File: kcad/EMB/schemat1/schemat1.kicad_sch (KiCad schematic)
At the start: 4 parts, among them IC1 ESP32-C6-WROOM-1-N8, U1 ER_OLEDM0.91_1x-I2C

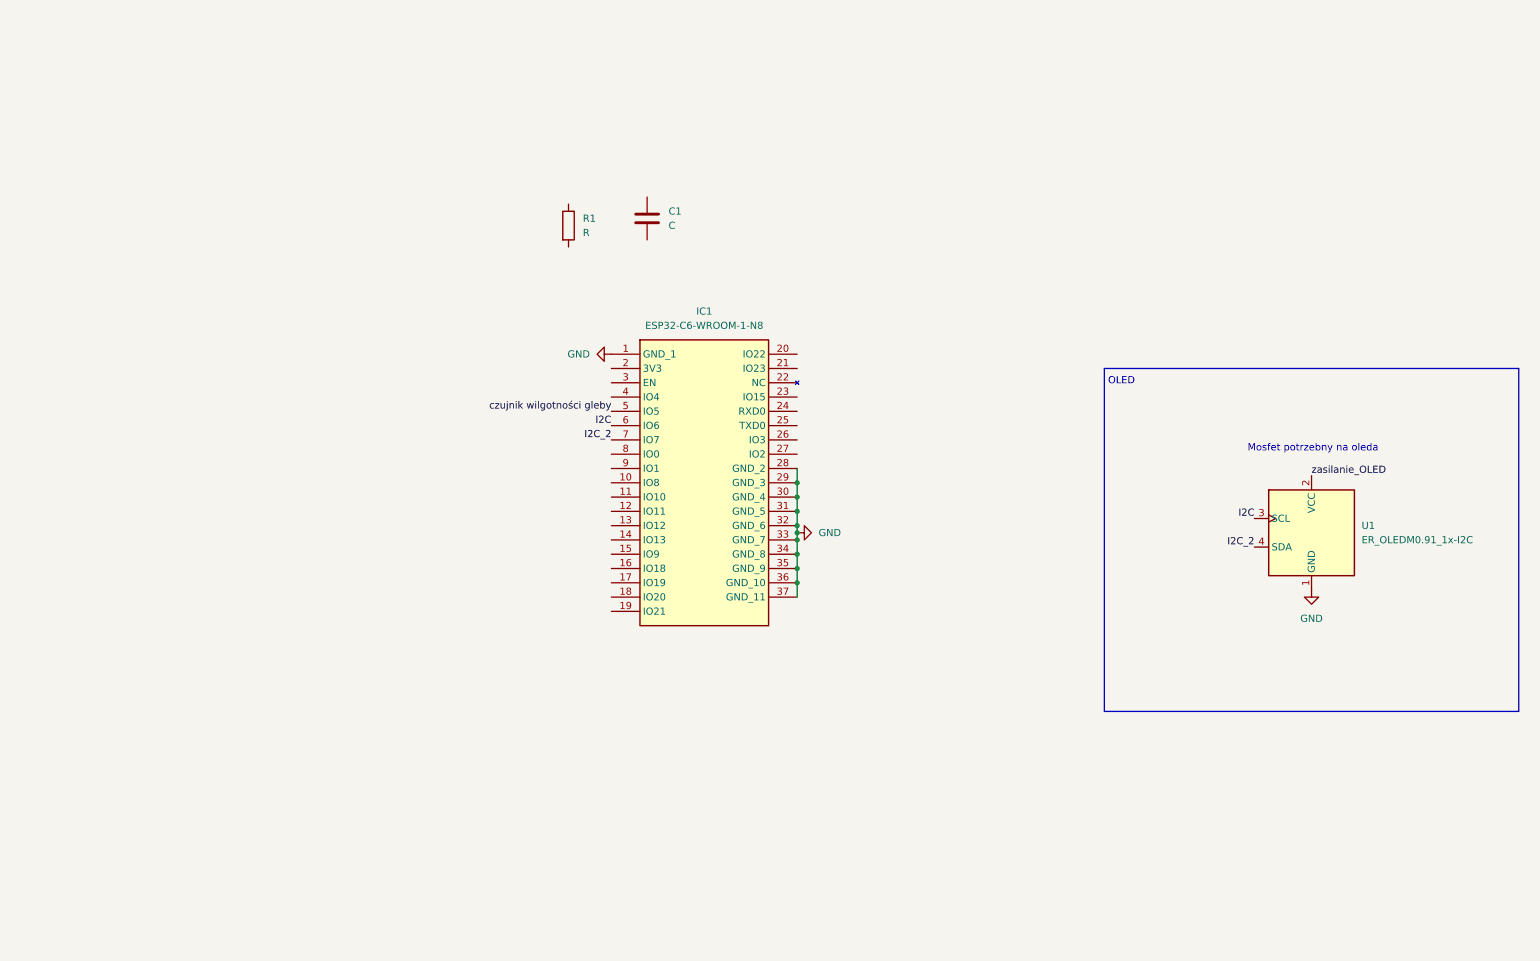
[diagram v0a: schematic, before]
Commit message: edit
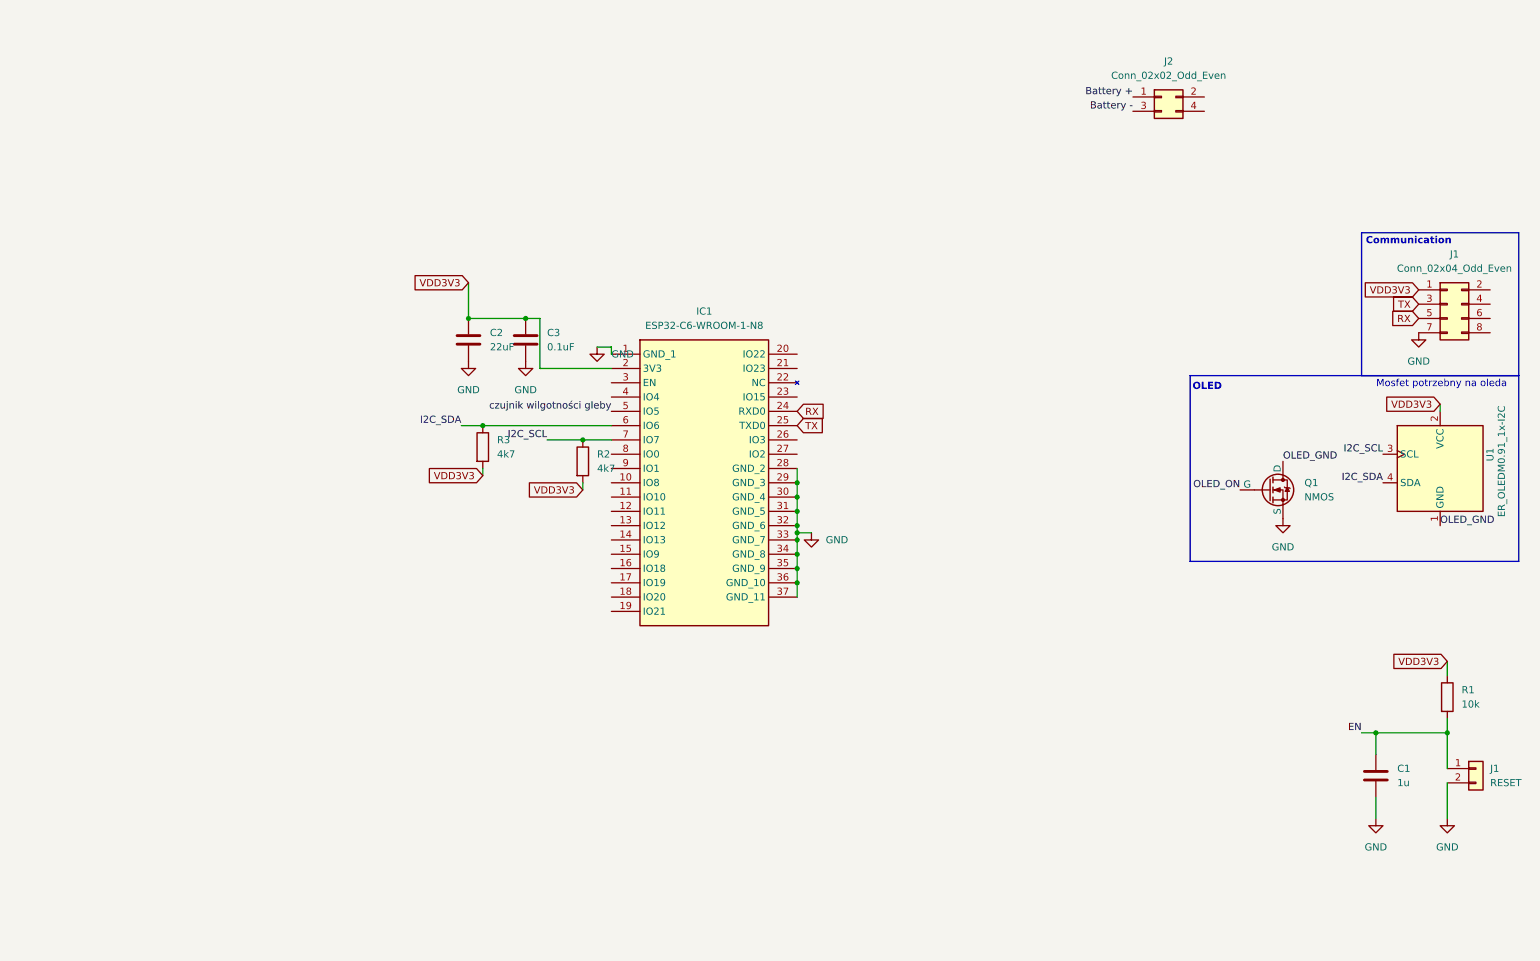
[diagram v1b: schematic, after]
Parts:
- added C2: 22uF, symbol Device:C
- added C3: 0.1uF, symbol Device:C
- added J1: RESET, symbol Connector_Generic:Conn_01x02
- added J1: Conn_02x04_Odd_Even, symbol Connector_Generic:Conn_02x04_Odd_Even
- added J2: Conn_02x02_Odd_Even, symbol Connector_Generic:Conn_02x02_Odd_Even
- added Q1: NMOS, symbol Simulation_SPICE:NMOS
- added R2, R3: 4k7, symbol Device:R
- C1: value C -> 1u
- R1: value R -> 10k
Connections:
- net zasilanie_OLED is gone; now on net VDD3V3: U1.2 (VCC)
- net GND: now also C1.2, C2.2, C3.2, J1.2 (Pin_2), J1.7 (Pin_7), Q1.3 (S); no longer U1.1 (GND)
- net VDD3V3: now reaches R1.1
- net VDD3V3: now also IC1.2 (3V3), C2.1, C3.1, J1.1 (Pin_1), R2.2, R3.2
- net EN: now reaches R1.2
- net EN: now also C1.1, J1.1 (Pin_1)
- net RX: now reaches IC1.24 (RXD0)
- net RX: now also J1.5 (Pin_5)
- net TX: now reaches IC1.25 (TXD0)
- net TX: now also J1.3 (Pin_3)
- net I2C renamed I2C_SCL
- net I2C_SCL: now also IC1.7 (IO7), R2.1; no longer IC1.6 (IO6)
- net I2C_2 renamed I2C_SDA
- net I2C_SDA: now also IC1.6 (IO6), R3.1; no longer IC1.7 (IO7)
- new net Battery +: J2.1 (Pin_1)
- new net Battery -: J2.3 (Pin_3)
- new net OLED_GND: Q1.1 (D), U1.1 (GND)
- new net OLED_ON: Q1.2 (G)
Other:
- note added: "Communication"
- moved on the sheet: U1

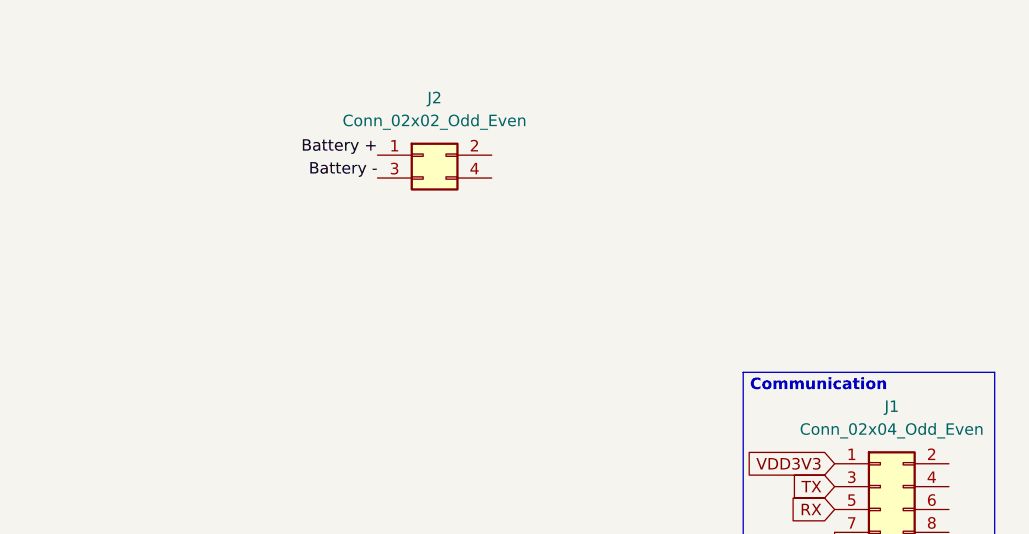
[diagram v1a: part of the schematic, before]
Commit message: update
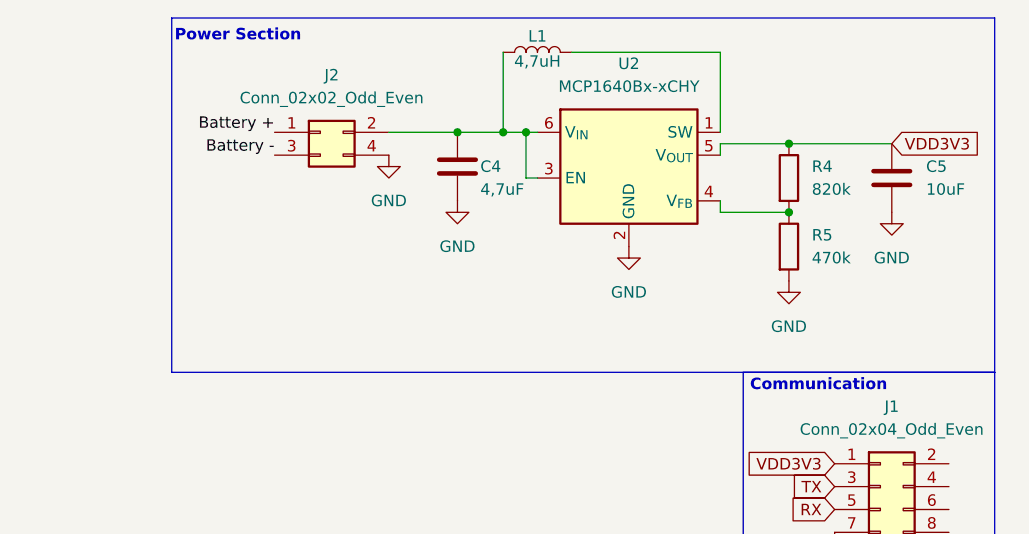
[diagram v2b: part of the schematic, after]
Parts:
- added C4: 4,7uF, symbol Device:C
- added C5: 10uF, symbol Device:C
- added L1: 4,7uH, symbol Device:L
- added R4: 820k, symbol Device:R
- added R5: 470k, symbol Device:R
- added U2: MCP1640Bx-xCHY, Package_TO_SOT_SMD:SOT-23-6, symbol Regulator_Switching:MCP1640Bx-xCHY
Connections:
- net GND: now also J2.4 (Pin_4), C4.2, C5.2, R5.2, U2.2 (GND)
- net VDD3V3: now also C5.1, R4.1, U2.5 (V_{OUT})
- net at J2.2 (Pin_2): now also C4.1, L1.1, U2.3 (EN), U2.6 (V_{IN})
- new net: R4.2, R5.1, U2.4 (V_{FB})
- new net: L1.2, U2.1 (SW)
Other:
- note added: "Power Section"
- moved on the sheet: J2

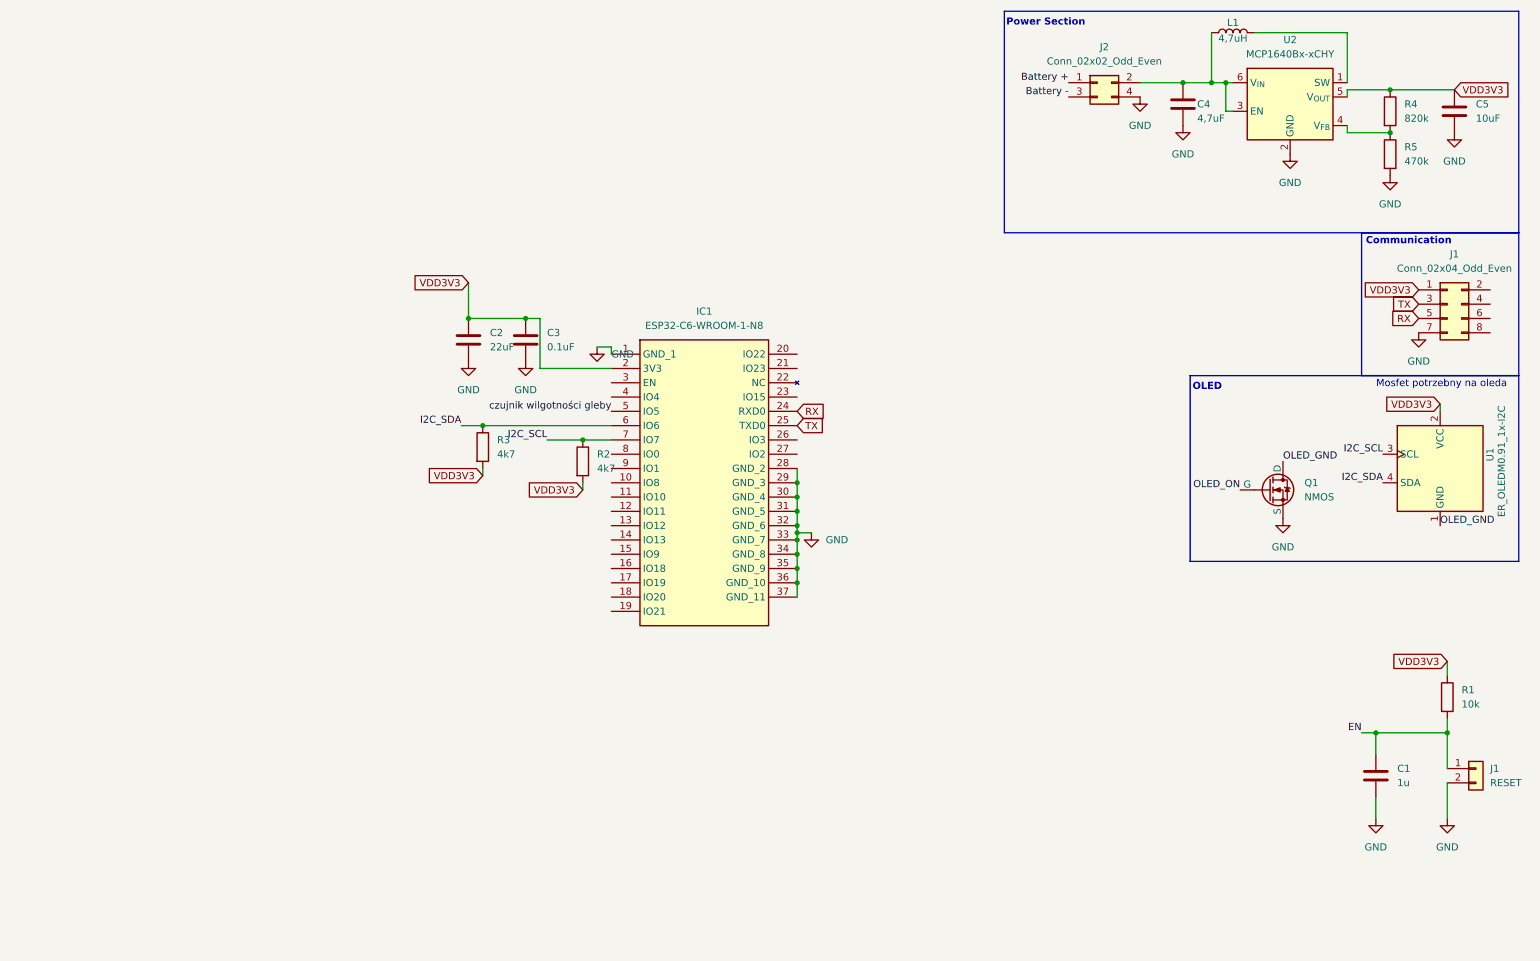
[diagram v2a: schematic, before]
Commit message: codes
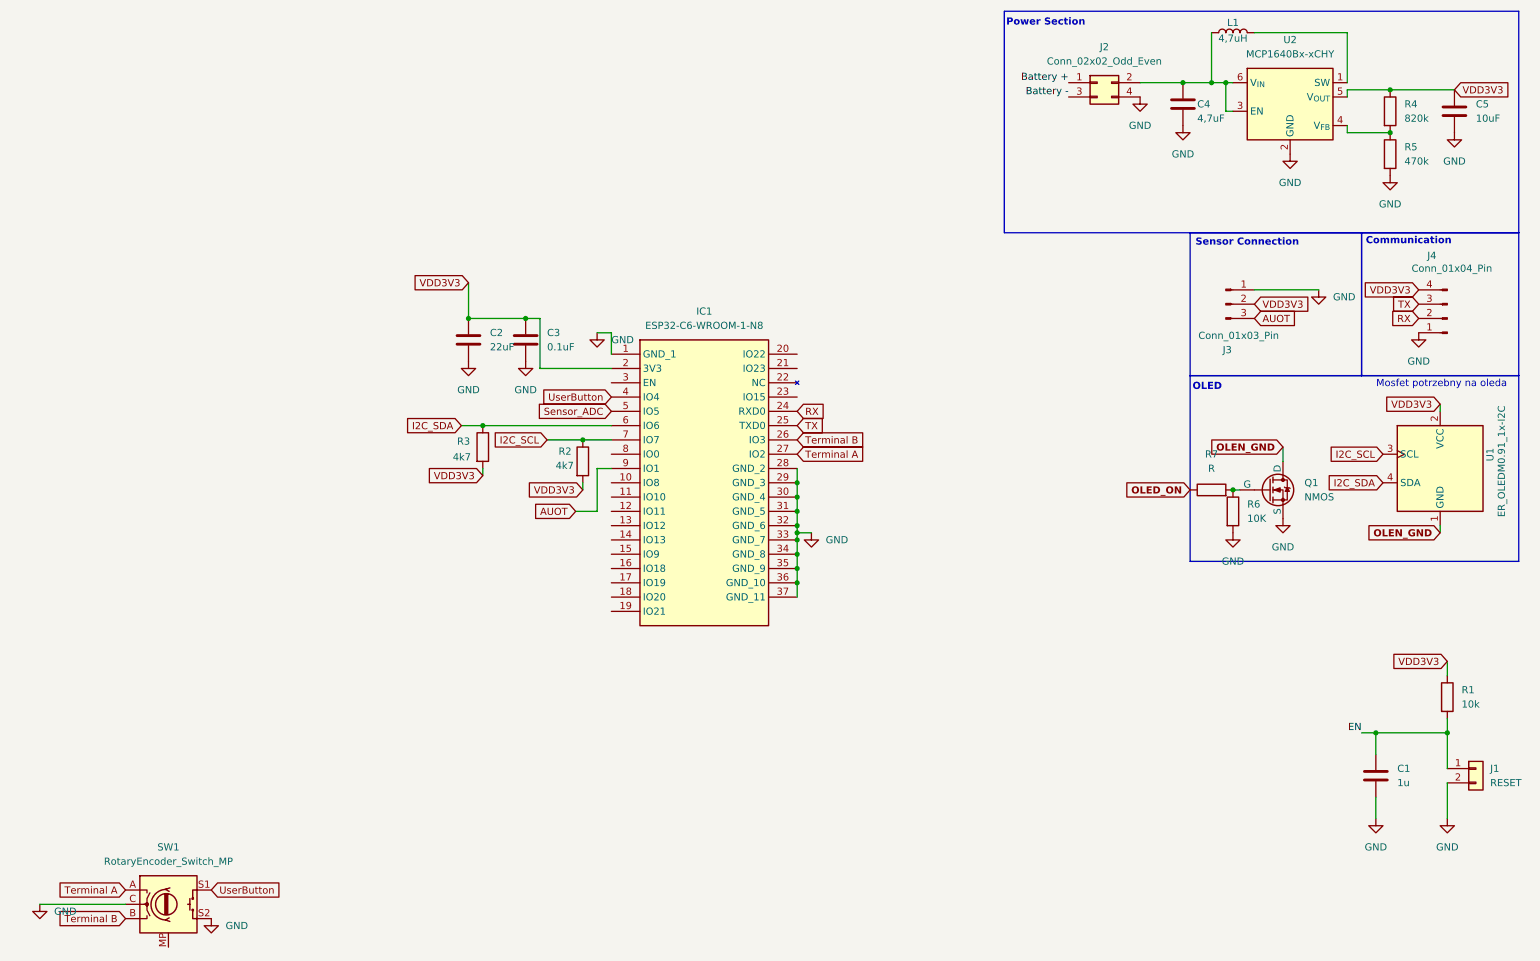
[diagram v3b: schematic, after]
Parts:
- removed J1: Conn_02x04_Odd_Even, symbol Connector_Generic:Conn_02x04_Odd_Even
- added J3: Conn_01x03_Pin, Connector_PinHeader_1.00mm:PinHeader_1x03_P1.00mm_Vertical, symbol Connector:Conn_01x03_Pin
- added J4: Conn_01x04_Pin, Connector_PinHeader_1.00mm:PinHeader_1x04_P1.00mm_Vertical, symbol Connector:Conn_01x04_Pin
- added R6: 10K, symbol Device:R
- added R7: R, symbol Device:R
- added SW1: RotaryEncoder_Switch_MP, Rotary_Encoder:RotaryEncoder_Alps_EC11E-Switch_Vertical_H20mm_MountingHoles, symbol Device:RotaryEncoder_Switch_MP
- Q1: footprint (none) -> Package_TO_SOT_SMD:TSOT-23
- U2: footprint Package_TO_SOT_SMD:SOT-23-6 -> (none)
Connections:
- net GND: now also J3.1 (Pin_1), J4.1 (Pin_1), R6.2, SW1.C, SW1.S2
- net OLED_ON: now also R7.1; no longer Q1.2 (G)
- net RX: now also J4.2 (Pin_2)
- net TX: now also J4.3 (Pin_3)
- net VDD3V3: now also J3.2 (Pin_2), J4.4 (Pin_4)
- net Terminal B: now reaches IC1.26 (IO3)
- net Terminal B: now also SW1.B
- net Terminal A: now reaches IC1.27 (IO2)
- net Terminal A: now also SW1.A
- net UserButton: now reaches IC1.4 (IO4)
- net UserButton: now also SW1.S1
- net AUOT: now reaches IC1.9 (IO1)
- net AUOT: now also J3.3 (Pin_3)
- net OLED_GND renamed OLEN_GND
- net czujnik wilgotności gleby renamed Sensor_ADC
- new net: Q1.2 (G), R6.1, R7.2
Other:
- note added: "Sensor Connection"

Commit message: schematic edit
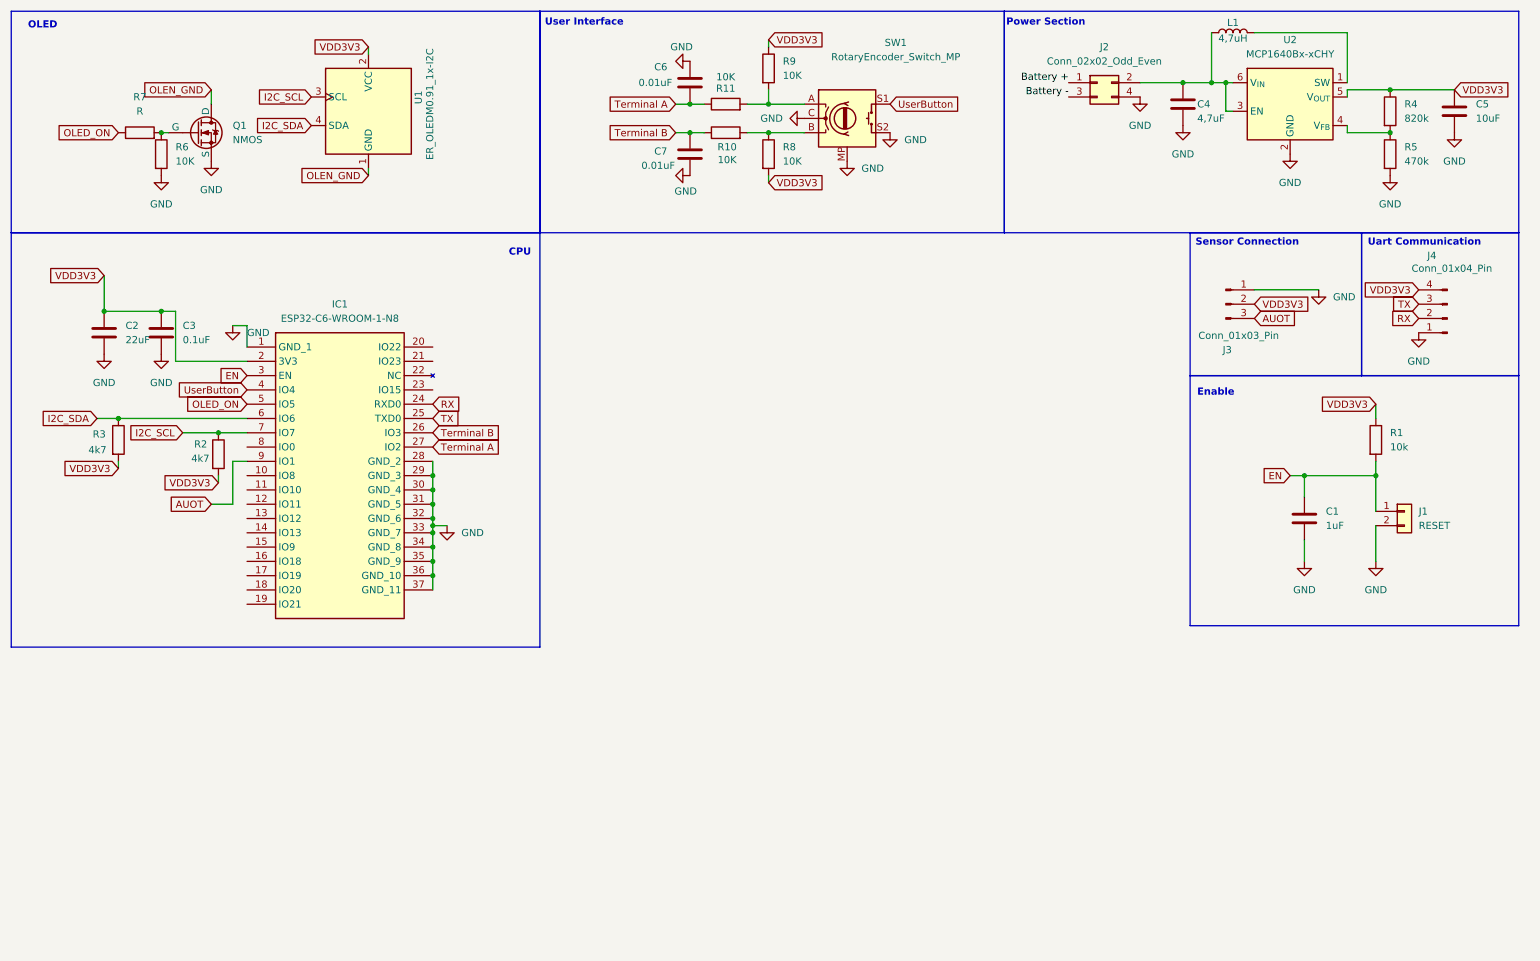
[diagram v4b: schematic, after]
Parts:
- added C6, C7: 0.01uF, symbol Device:C
- added R10, R11, R8, R9: 10K, symbol Device:R
- C1: value 1u -> 1uF
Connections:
- net Sensor_ADC is gone; now on net OLED_ON: IC1.5 (IO5)
- net EN: now also IC1.3 (EN)
- net GND: now also SW1.MP, C6.1, C7.2
- net Terminal A: now also C6.2, R11.1; no longer SW1.A
- net Terminal B: now also C7.1, R10.1; no longer SW1.B
- net VDD3V3: now also R8.2, R9.1
- new net: R11.2, R9.2, SW1.A
- new net: R10.2, R8.1, SW1.B
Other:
- note added: "CPU"
- note added: "Enable"
- note added: "Uart Communication"
- note added: "User Interface"
- note removed: "Communication"
- note removed: "Mosfet potrzebny na oleda"
- moved on the sheet: C1, C2, C3, IC1, J1, Q1, R1, R2, R3, R6, R7, SW1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
